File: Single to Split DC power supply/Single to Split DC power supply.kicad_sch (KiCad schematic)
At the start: 46 parts, among them J1 Conn_01x02, J2 Conn_01x02, J3 Conn_01x02, J4 Conn_01x02, Q1 AO3401A, Q2 AO3401A, U1 TPS5430DDA, U2 TPS65131RGER

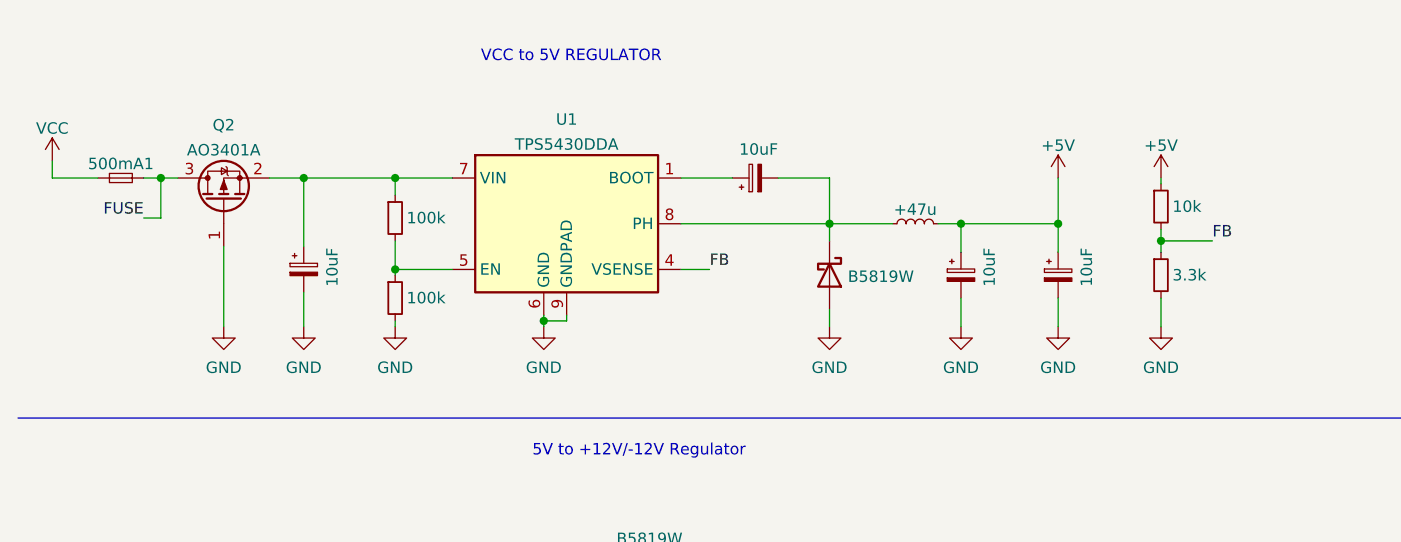
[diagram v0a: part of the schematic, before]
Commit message: Add files via upload
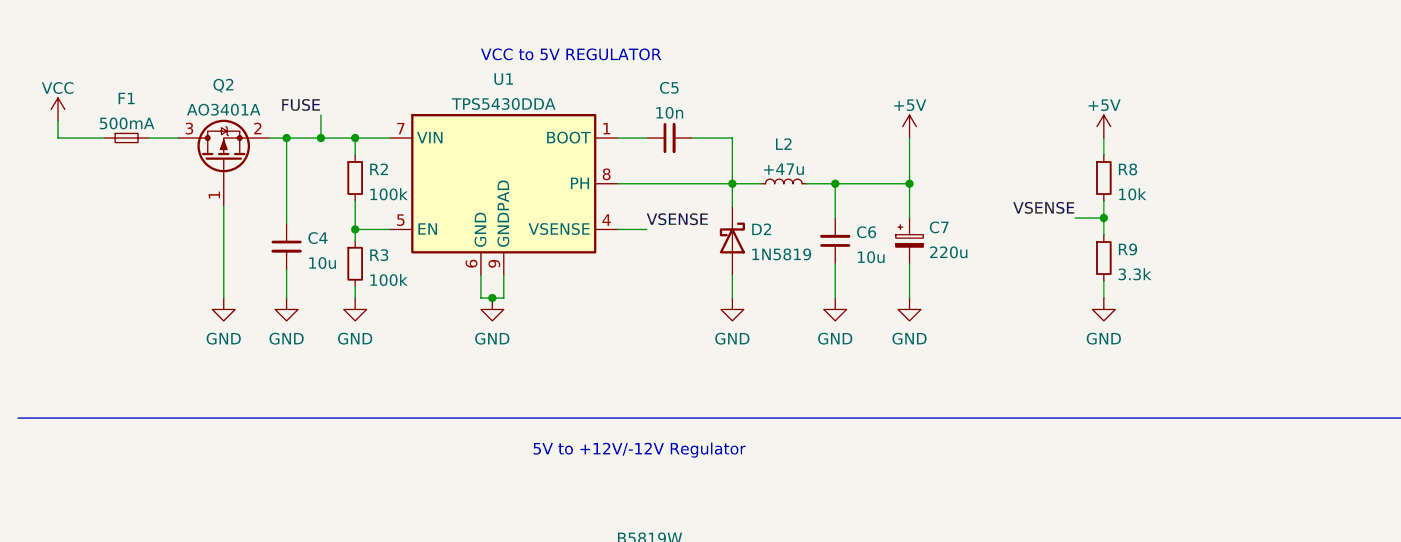
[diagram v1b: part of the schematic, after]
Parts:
- removed 500mA1: Fuse_Small, symbol Device:Fuse_Small
- removed c1, c2, c3, c4: 10uF, symbol Device:C_Polarized_Small
- added C4, C6: 10u, Capacitor_SMD:C_0603_1608Metric, symbol Device:C_Small
- added C5: 10n, Capacitor_SMD:C_0603_1608Metric, symbol Device:C_Small
- added C7: 220u, Capacitor_SMD:CP_Elec_4x5.4, symbol Device:C_Polarized_Small
- added F1: 500mA, Package_DIP:SMDIP-4_W9.53mm, symbol Device:Fuse_Small
- C1, C2, C3: footprint (none) -> Capacitor_SMD:C_0603_1608Metric
- C10: renamed from C6; footprint (none) -> Capacitor_SMD:C_0603_1608Metric
- C11: renamed from C7; footprint (none) -> Capacitor_SMD:C_0603_1608Metric
- C12: renamed from C8; footprint (none) -> Capacitor_SMD:C_0603_1608Metric
- C13: renamed from C9; footprint (none) -> Capacitor_SMD:C_0603_1608Metric
- C8: renamed from C4; footprint (none) -> Capacitor_SMD:C_0603_1608Metric
- C9: renamed from C5; footprint (none) -> Capacitor_SMD:C_0603_1608Metric
- D2: value B5819W -> 1N5819
- D4, D5, D6, D7: footprint (none) -> LED_SMD:LED_1206_3216Metric
- H1, H2, H3, H4: footprint (none) -> MountingHole:MountingHole_3.2mm_M3_Pad_Via
- J1, J2, J3, J4: footprint (none) -> TerminalBlock:TerminalBlock_Altech_AK300-2_P5.00mm
- L1, L2, L3: footprint (none) -> Inductor_SMD:L_1206_3216Metric
- R1, R10, R2, R3, R4, R5, R6, R7, R8, R9: footprint (none) -> Resistor_SMD:R_0603_1608Metric
- U2: footprint RGE0024B -> TPS65131RGER:RGE0024B
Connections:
- net +5V: now also C6.2, C7.1
- net FUSE: now also Q2.2 (S), R2.1, U1.7 (VIN), C4.1; no longer Q2.3 (D)
- net GND: now also C4.2, C6.1, C7.2
- net VCC: now also F1.1
- net at D2.1 (K), L2.1, U1.8 (PH): now also C5.2
- net at U1.1 (BOOT): now also C5.1
- net FB renamed VSENSE
- new net: F1.2, Q2.3 (D)
